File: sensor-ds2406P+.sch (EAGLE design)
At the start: 14 parts, among them IC1 DS2406P+

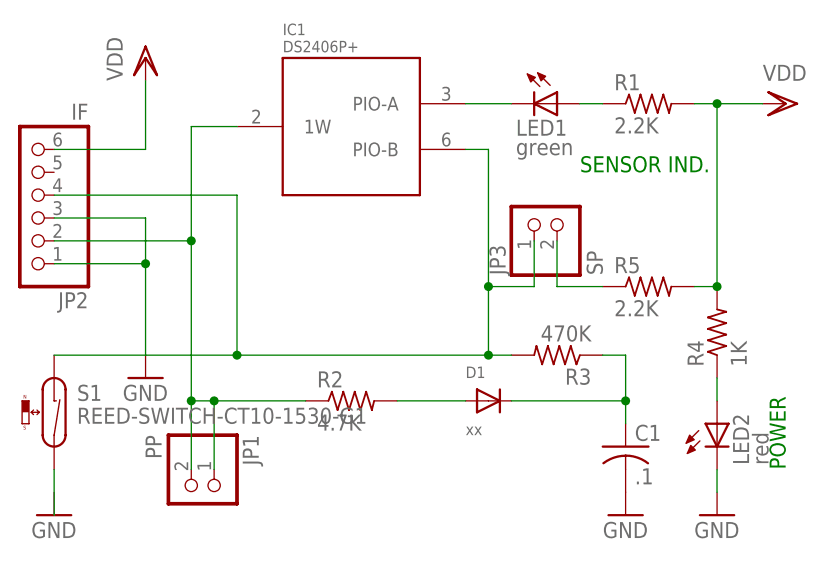
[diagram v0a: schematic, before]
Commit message: Add files via upload
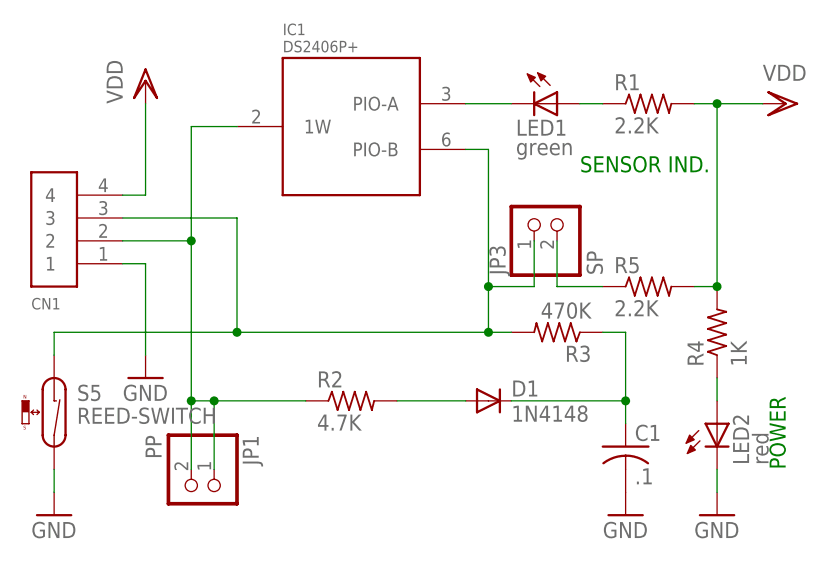
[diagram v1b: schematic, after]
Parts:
- removed JP2: IF, adafruit:PINHD-1X6
- removed S1: REED-SWITCH-CT10-1530-G1, switch-reed:REED-SWITCH-CT10-1530-G1
- added CN1: 1X4-BIG, adafruit:1X4-BIG
- added S5: REED-SWITCH, switch-reed:REED-SWITCH-MK15-C2
- D1: value xx -> 1N4148; device adafruit:DIODESOD-123 -> dont:MMBF1N4148MMBD4148
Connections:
- net GND: now also CN1.1, S5.2; no longer JP2.1, JP2.3, S1.2
- net IO: now also CN1.2; no longer JP2.2
- net PIO$B: now also CN1.3, S5.1; no longer JP2.4, S1.1
- net VDD: now also CN1.4; no longer JP2.6
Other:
- moved on the sheet: R3
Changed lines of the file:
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@@
 <classes>
 <class number="0" name="default" width="0" drill="0">
+<clearance class="0" value="0.205"/>
 </class>
 </classes>
@@
 <part name="R4" library="resistor" deviceset="R-US_" device="R0805" value="1K"/>
 <part name="R5" library="resistor" deviceset="R-US_" device="R0805" value="2.2K"/>
-<part name="JP2" library="adafruit" deviceset="PINHD-1X6" device="" value="IF"/>
 <part name="R1" library="rcl" deviceset="R-US_" device="R0805" value="2.2K"/>
 <part name="R2" library="rcl" deviceset="R-US_" device="R0805" value="4.7K"/>
-<part name="D1" library="adafruit" deviceset="DIODE" device="SOD-123" value="xx"/>
 <part name="JP1" library="pinhead" deviceset="PINHD-1X2" device="" value="PP"/>
 <part name="JP3" library="pinhead" deviceset="PINHD-1X2" device="" value="SP"/>
 <part name="IC1" library="dont" deviceset="DS2406P+" device=""/>
-<part name="S1" library="switch-reed" deviceset="REED-SWITCH-" device="CT10-1530-G1"/>
 <part name="GND4" library="supply1" deviceset="GND" device=""/>
+<part name="S5" library="switch-reed" deviceset="REED-SWITCH-" device="MK15-C2" value="REED-SWITCH"/>
+<part name="CN1" library="adafruit" deviceset="1X4" device="-BIG" value=""/>
+<part name="D1" library="dont" deviceset="MMBF1N4148" device="MMBD4148" value="1N4148"/>
 </parts>
 <sheets>
@@
 <instance part="GND1" gate="1" x="106.68" y="139.7"/>
 <instance part="GND2" gate="1" x="160.02" y="124.46"/>
-<instance part="R3" gate="G$1" x="152.4" y="142.24" rot="R180"/>
+<instance part="R3" gate="G$1" x="152.4" y="144.78" rot="R180"/>
 <instance part="GND3" gate="1" x="170.18" y="124.46"/>
-<instance part="VDD1" gate="G$1" x="106.68" y="175.26"/>
+<instance part="VDD1" gate="G$1" x="106.68" y="172.72"/>
 <instance part="VDD2" gate="G$1" x="177.8" y="170.18" rot="R270"/>
 <instance part="FRAME1" gate="G$1" x="12.7" y="48.26"/>
@@
 <instance part="R4" gate="G$1" x="170.18" y="144.78" rot="R90"/>
 <instance part="R5" gate="G$1" x="162.56" y="149.86"/>
-<instance part="JP2" gate="A" x="93.98" y="160.02" rot="R180"/>
 <instance part="R1" gate="G$1" x="162.56" y="170.18"/>
 <instance part="R2" gate="G$1" x="129.54" y="137.16"/>
-<instance part="D1" gate="G$1" x="144.78" y="137.16"/>
 <instance part="JP1" gate="G$1" x="111.76" y="127" rot="R270"/>
 <instance part="JP3" gate="G$1" x="152.4" y="157.48" rot="R90"/>
 <instance part="IC1" gate="G$1" x="129.54" y="167.64"/>
-<instance part="S1" gate="G$1" x="96.52" y="134.62"/>
 <instance part="GND4" gate="1" x="96.52" y="124.46"/>
+<instance part="S5" gate="G$1" x="96.52" y="134.62"/>
+<instance part="CN1" gate="G$1" x="99.06" y="154.94" rot="R180"/>
+<instance part="D1" gate="1" x="144.78" y="137.16"/>
 </instances>
 <busses>
@@
 <net name="GND" class="0">
 <segment>
-<wire x1="96.52" y1="152.4" x2="106.68" y2="152.4" width="0.1524" layer="91"/>
+<wire x1="104.14" y1="152.4" x2="106.68" y2="152.4" width="0.1524" layer="91"/>
 <pinref part="GND1" gate="1" pin="GND"/>
 <wire x1="106.68" y1="152.4" x2="106.68" y2="142.24" width="0.1524" layer="91"/>
-<wire x1="96.52" y1="157.48" x2="106.68" y2="157.48" width="0.1524" layer="91"/>
-<wire x1="106.68" y1="157.48" x2="106.68" y2="152.4" width="0.1524" layer="91"/>
-<junction x="106.68" y="152.4"/>
-<pinref part="JP2" gate="A" pin="1"/>
-<pinref part="JP2" gate="A" pin="3"/>
+<pinref part="CN1" gate="G$1" pin="1"/>
 </segment>
 <segment>
@@
 </segment>
 <segment>
-<pinref part="S1" gate="G$1" pin="2"/>
-<wire x1="96.52" y1="129.54" x2="96.52" y2="124.46" width="0.1524" layer="91"/>
+<pinref part="S5" gate="G$1" pin="2"/>
+<pinref part="GND4" gate="1" pin="GND"/>
+<wire x1="96.52" y1="129.54" x2="96.52" y2="127" width="0.1524" layer="91"/>
 </segment>
 </net>
@@
 <wire x1="142.24" y1="137.16" x2="134.62" y2="137.16" width="0.1524" layer="91"/>
 <pinref part="R2" gate="G$1" pin="2"/>
-<pinref part="D1" gate="G$1" pin="A"/>
+<pinref part="D1" gate="1" pin="A"/>
 </segment>
 </net>
 <net name="PIO$B" class="0">
 <segment>
-<wire x1="116.84" y1="142.24" x2="116.84" y2="160.02" width="0.1524" layer="91"/>
-<wire x1="116.84" y1="160.02" x2="96.52" y2="160.02" width="0.1524" layer="91"/>
-<pinref part="JP2" gate="A" pin="4"/>
+<wire x1="116.84" y1="144.78" x2="116.84" y2="157.48" width="0.1524" layer="91"/>
+<wire x1="116.84" y1="157.48" x2="104.14" y2="157.48" width="0.1524" layer="91"/>
 <pinref part="R3" gate="G$1" pin="2"/>
-<wire x1="147.32" y1="142.24" x2="144.78" y2="142.24" width="0.1524" layer="91"/>
+<wire x1="147.32" y1="144.78" x2="144.78" y2="144.78" width="0.1524" layer="91"/>
 <pinref part="JP3" gate="G$1" pin="1"/>
 <wire x1="144.78" y1="165.1" x2="144.78" y2="149.86" width="0.1524" layer="91"/>
@@
 <wire x1="149.86" y1="149.86" x2="144.78" y2="149.86" width="0.1524" layer="91"/>
 <junction x="144.78" y="149.86"/>
-<wire x1="144.78" y1="149.86" x2="144.78" y2="142.24" width="0.1524" layer="91"/>
-<wire x1="116.84" y1="142.24" x2="144.78" y2="142.24" width="0.1524" layer="91"/>
-<junction x="144.78" y="142.24"/>
+<wire x1="144.78" y1="149.86" x2="144.78" y2="144.78" width="0.1524" layer="91"/>
+<wire x1="116.84" y1="144.78" x2="144.78" y2="144.78" width="0.1524" layer="91"/>
+<junction x="144.78" y="144.78"/>
 <pinref part="IC1" gate="G$1" pin="PIO-B"/>
 <wire x1="144.78" y1="165.1" x2="142.24" y2="165.1" width="0.1524" layer="91"/>
-<pinref part="S1" gate="G$1" pin="1"/>
-<wire x1="116.84" y1="142.24" x2="96.52" y2="142.24" width="0.1524" layer="91"/>
-<junction x="116.84" y="142.24"/>
+<wire x1="116.84" y1="144.78" x2="96.52" y2="144.78" width="0.1524" layer="91"/>
+<junction x="116.84" y="144.78"/>
+<wire x1="96.52" y1="144.78" x2="96.52" y2="142.24" width="0.1524" layer="91"/>
+<pinref part="S5" gate="G$1" pin="1"/>
+<pinref part="CN1" gate="G$1" pin="3"/>
 </segment>
 </net>
 <net name="VDD" class="0">
 <segment>
-<wire x1="96.52" y1="165.1" x2="106.68" y2="165.1" width="0.1524" layer="91"/>
-<wire x1="106.68" y1="165.1" x2="106.68" y2="172.72" width="0.1524" layer="91"/>
+<wire x1="104.14" y1="160.02" x2="106.68" y2="160.02" width="0.1524" layer="91"/>
+<wire x1="106.68" y1="160.02" x2="106.68" y2="170.18" width="0.1524" layer="91"/>
 <pinref part="VDD1" gate="G$1" pin="VDD"/>
-<pinref part="JP2" gate="A" pin="6"/>
+<pinref part="CN1" gate="G$1" pin="4"/>
 </segment>
 <segment>
@@
 <segment>
 <pinref part="R3" gate="G$1" pin="1"/>
-<wire x1="160.02" y1="142.24" x2="157.48" y2="142.24" width="0.1524" layer="91"/>
+<wire x1="160.02" y1="144.78" x2="157.48" y2="144.78" width="0.1524" layer="91"/>
 <wire x1="147.32" y1="137.16" x2="160.02" y2="137.16" width="0.1524" layer="91"/>
 <wire x1="160.02" y1="134.62" x2="160.02" y2="137.16" width="0.1524" layer="91"/>
-<wire x1="160.02" y1="137.16" x2="160.02" y2="142.24" width="0.1524" layer="91"/>
+<wire x1="160.02" y1="137.16" x2="160.02" y2="144.78" width="0.1524" layer="91"/>
 <pinref part="C1" gate="G$1" pin="1"/>
 <junction x="160.02" y="137.16"/>
-<pinref part="D1" gate="G$1" pin="C"/>
+<pinref part="D1" gate="1" pin="C"/>
 </segment>
 </net>
@@
 <net name="IO" class="0">
 <segment>
-<wire x1="96.52" y1="154.94" x2="111.76" y2="154.94" width="0.1524" layer="91"/>
+<wire x1="104.14" y1="154.94" x2="111.76" y2="154.94" width="0.1524" layer="91"/>
 <wire x1="111.76" y1="154.94" x2="111.76" y2="167.64" width="0.1524" layer="91"/>
 <wire x1="111.76" y1="167.64" x2="116.84" y2="167.64" width="0.1524" layer="91"/>
-<pinref part="JP2" gate="A" pin="2"/>
 <pinref part="JP1" gate="G$1" pin="2"/>
 <wire x1="111.76" y1="154.94" x2="111.76" y2="137.16" width="0.1524" layer="91"/>
@@
 <junction x="111.76" y="137.16"/>
 <junction x="114.3" y="137.16"/>
+<pinref part="CN1" gate="G$1" pin="2"/>
 </segment>
 </net>
